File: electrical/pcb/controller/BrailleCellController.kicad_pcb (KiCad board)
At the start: 2 copper layers, 7 x 12 mm, 4 parts, among them J1 Conn_01x08_Socket, J2 Conn_01x08_Socket, J5 Conn_01x05_Socket, U1 HV509K6-G

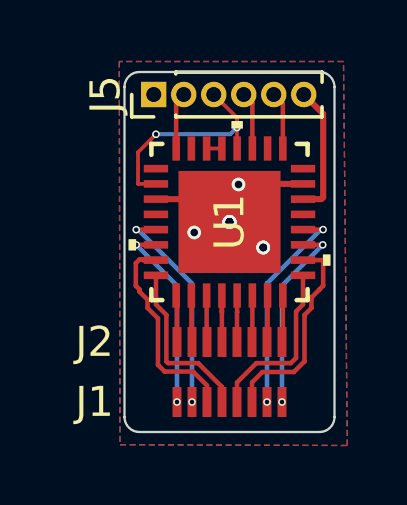
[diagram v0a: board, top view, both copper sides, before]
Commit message: library fix
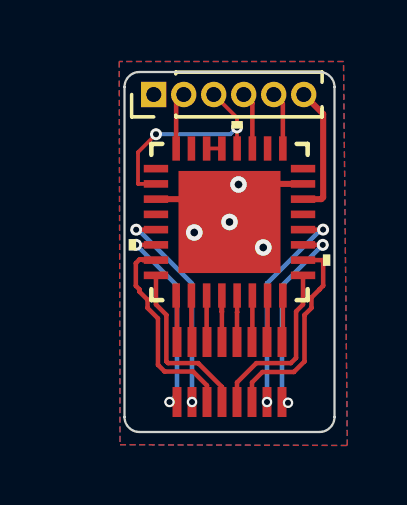
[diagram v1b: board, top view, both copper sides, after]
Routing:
- net GND: vias 10 -> 4
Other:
- board text added: "CONTROLLER"
